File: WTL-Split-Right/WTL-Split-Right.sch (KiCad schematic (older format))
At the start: 46 parts, among them J1 MJ-4PP-9, U1 ProMicro

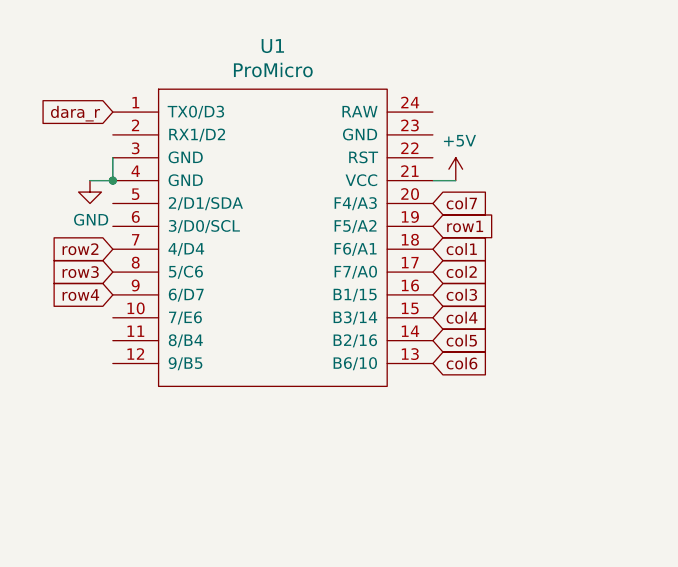
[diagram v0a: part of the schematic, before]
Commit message: i'm fucking tired
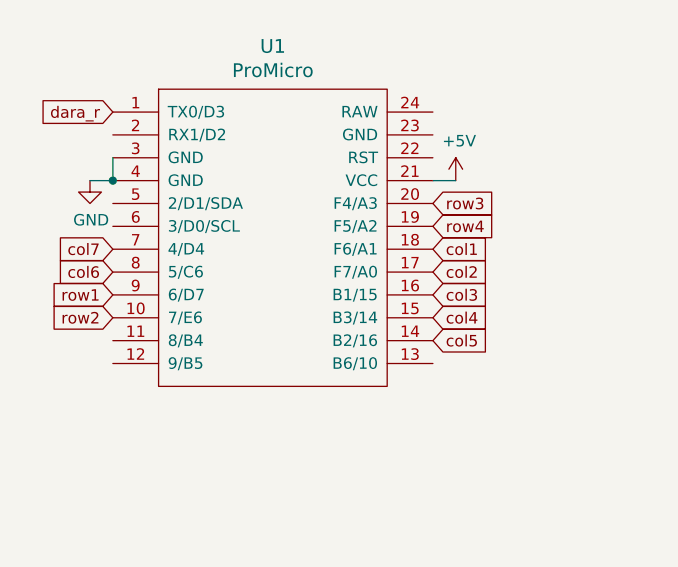
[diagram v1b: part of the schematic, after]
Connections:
- net col6: now also U1.8 (5/C6); no longer U1.13 (B6/10)
- net col7: now also U1.7 (4/D4); no longer U1.20 (F4/A3)
- net row1: now also U1.9 (6/D7); no longer U1.19 (F5/A2)
- net row2: now also U1.10 (7/E6); no longer U1.7 (4/D4)
- net row3: now also U1.20 (F4/A3); no longer U1.8 (5/C6)
- net row4: now also U1.19 (F5/A2); no longer U1.9 (6/D7)
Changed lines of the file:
@@
 Text GLabel 2700 2950 0    50   Input ~ 0
 dara_r
-Text GLabel 4100 3350 2    50   Input ~ 0
+Text GLabel 2700 3550 0    50   Input ~ 0
 col7
-Text GLabel 4100 4050 2    50   Input ~ 0
+Text GLabel 2700 3650 0    50   Input ~ 0
 col6
 Text GLabel 4100 3950 2    50   Input ~ 0
@@
 Text GLabel 4100 3550 2    50   Input ~ 0
 col1
+Text GLabel 2700 3750 0    50   Input ~ 0
+row1
+Text GLabel 2700 3850 0    50   Input ~ 0
+row2
+Text GLabel 4100 3350 2    50   Input ~ 0
+row3
 Text GLabel 4100 3450 2    50   Input ~ 0
-row1
-Text GLabel 2700 3550 0    50   Input ~ 0
-row2
-Text GLabel 2700 3650 0    50   Input ~ 0
-row3
-Text GLabel 2700 3750 0    50   Input ~ 0
 row4
 $EndSCHEMATC

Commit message: I don't remember what i've done
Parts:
- J1: symbol kbd:MJ-4PP-9 -> WTL-Split-Right-rescue:MJ-4PP-9-kbd
- MX21: footprint MX_Only:MXOnly-2U-NoLED -> MX_Only:MXOnly-2U-ReversedStabilizers-NoLED
- U1: symbol kbd:ProMicro -> WTL-Split-Right-rescue:ProMicro-kbd
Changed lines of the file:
@@
 F 0 "MX21" H 6633 4723 60  0000 C CNN
 F 1 "MX-NoLED" H 6633 4649 20  0000 C CNN
-F 2 "MX_Only:MXOnly-2U-NoLED" H 5975 4475 60  0001 C CNN
+F 2 "MX_Only:MXOnly-2U-ReversedStabilizers-NoLED" H 5975 4475 60  0001 C CNN
 F 3 "" H 5975 4475 60  0001 C CNN
 	1    6600 4500
@@
 col7
 $Comp
-L kbd:ProMicro U1
+L WTL-Split-Right-rescue:ProMicro-kbd U1
 U 1 1 613E4DD7
 P 3400 3500
@@
 $EndComp
 $Comp
-L kbd:MJ-4PP-9 J1
+L WTL-Split-Right-rescue:MJ-4PP-9-kbd J1
 U 1 1 613E65F2
 P 3900 2100
